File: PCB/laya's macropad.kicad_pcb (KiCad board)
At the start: 2 copper layers, 47.1 x 65.3 mm, 10 parts, among them J1 OLED_128x64, U2 MCU_Seeed_XIAO_RP2040

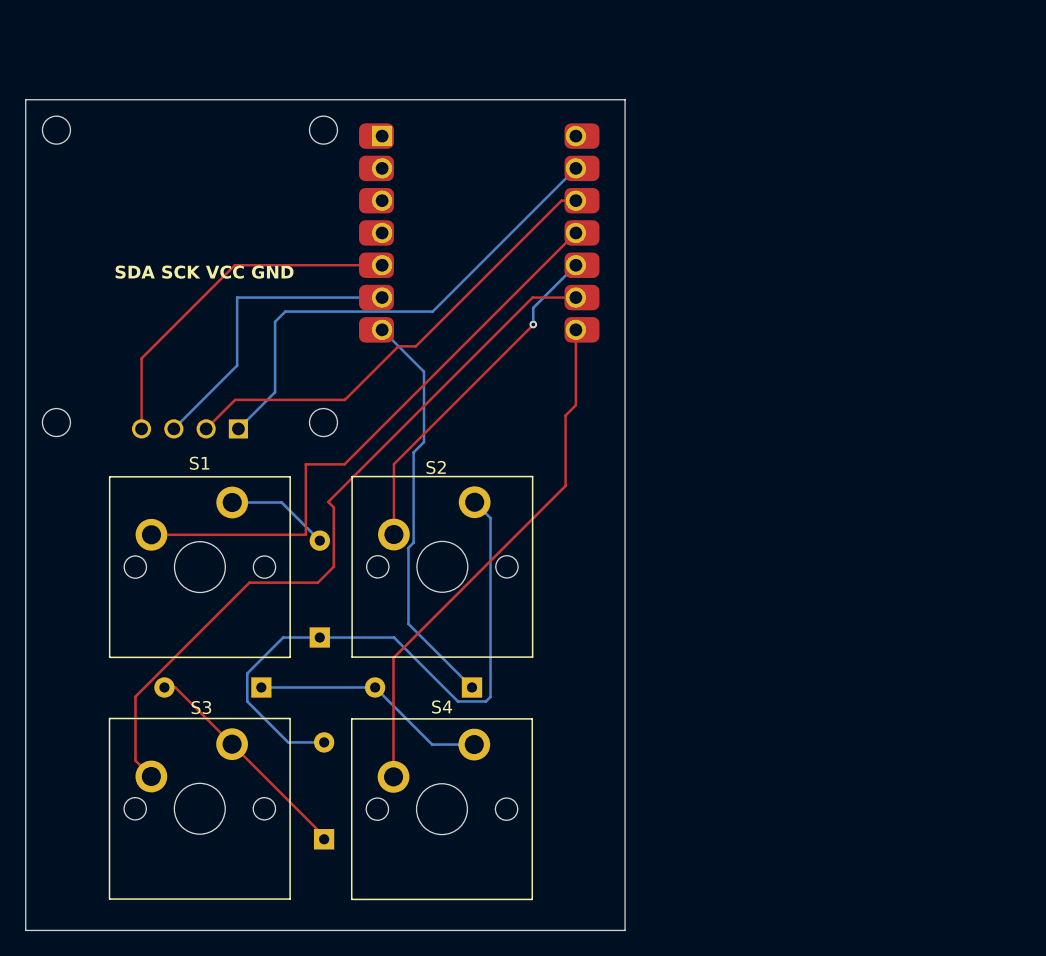
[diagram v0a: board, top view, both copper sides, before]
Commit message: oled changed
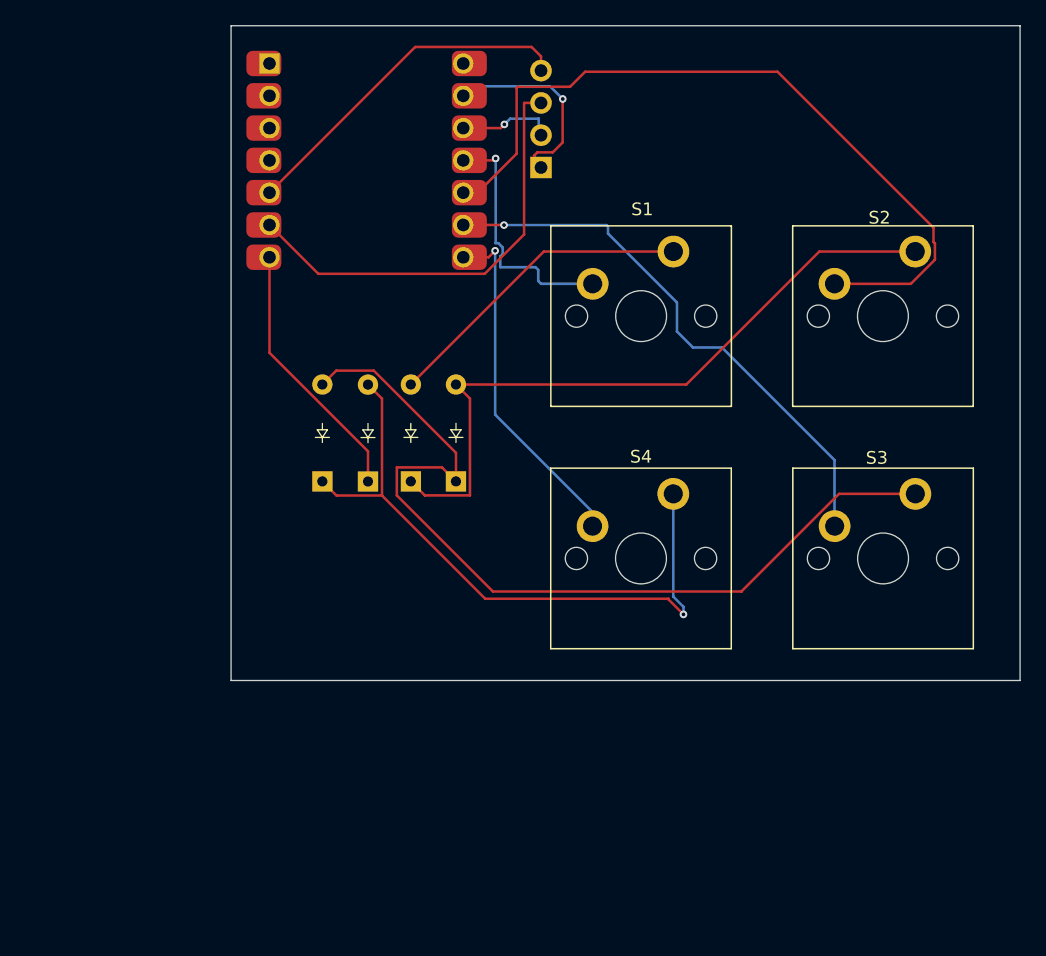
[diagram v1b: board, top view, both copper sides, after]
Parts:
- D1, D2, D3, D4: moved to F.Cu
- J1: value OLED_128x64 -> OLED_128x32; footprint ScottoKeebs_Components:OLED_128x64 -> ScottoKeebs_Components:OLED_128x32
- moved S3 57.2 mm to (183.0, 88.0)
- moved S1 39.9 mm to (164.0, 68.9)
- moved S2 39.9 mm to (183.0, 68.9)
- moved J1 31.8 mm to (154.5, 47.4)
- moved D2 30.0 mm to (149.4, 81.9)
- moved S4 25.2 mm to (164.0, 88.0)
- moved D4 18.1 mm to (142.5, 81.9), turned to 90 degrees
- moved D3 16.9 mm to (138.9, 81.9), turned to 90 degrees
- moved D1 14.2 mm to (145.8, 81.9)
- moved U2 10.5 mm to (142.4, 56.6)
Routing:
- net Net-(D2-K): track 17.6 -> 70.3 mm
- net Net-(U2-PA5_A9_D9_MISO): track 27.1 -> 60.3 mm, vias 1 -> 0
- net Net-(D3-K): track 18.6 -> 51.8 mm, vias 0 -> 1
- net Net-(J1-VCC): track 36.5 -> 7.62 mm, vias 0 -> 1
- net Net-(U2-PA6_A10_D10_MOSI): track 46.5 -> 19.9 mm, vias 0 -> 1
- net GND: track 38.3 -> 15.8 mm, vias 0 -> 1
- net Net-(D1-A): track 8.13 -> 25.0 mm
- net Net-(U2-PB09_A7_D7_RX): track 41.1 -> 25.8 mm, vias 0 -> 1
- net Net-(U2-PA7_A8_D8_SCK): track 58.0 -> 43.7 mm, vias 0 -> 1
- net Net-(D4-K): track 32.1 -> 20.8 mm
- net Net-(J1-SCL): track 23.8 -> 34.8 mm
- net Net-(D1-K): track 47.9 -> 54.7 mm
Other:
- board size 47.1 x 65.3 mm -> 62.1 x 51.5 mm
